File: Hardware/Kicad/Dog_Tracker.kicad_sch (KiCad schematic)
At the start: 20 parts, among them IC1 M4 Feather, U1 ADP160AUJZ-1.8-R7, U2 SX1280IMLTRT, U3 Origin_GPS1510, U4 NFA18SL407V1A45L, U5 SN74AUP1T97, U6 LSM6DSO32

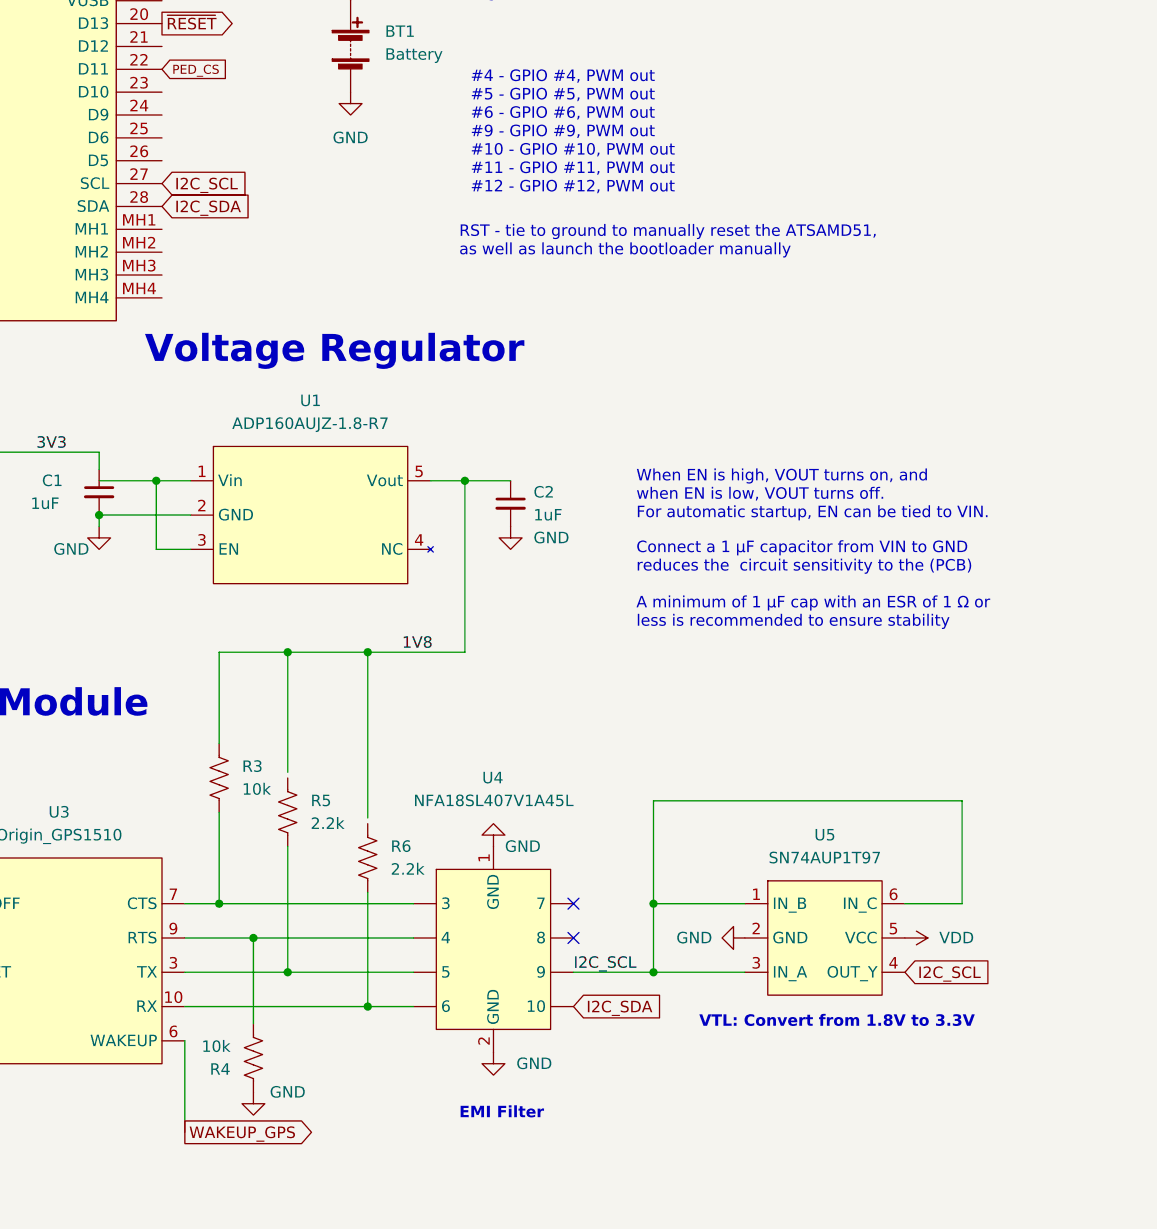
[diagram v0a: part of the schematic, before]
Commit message: 'wire i2c'
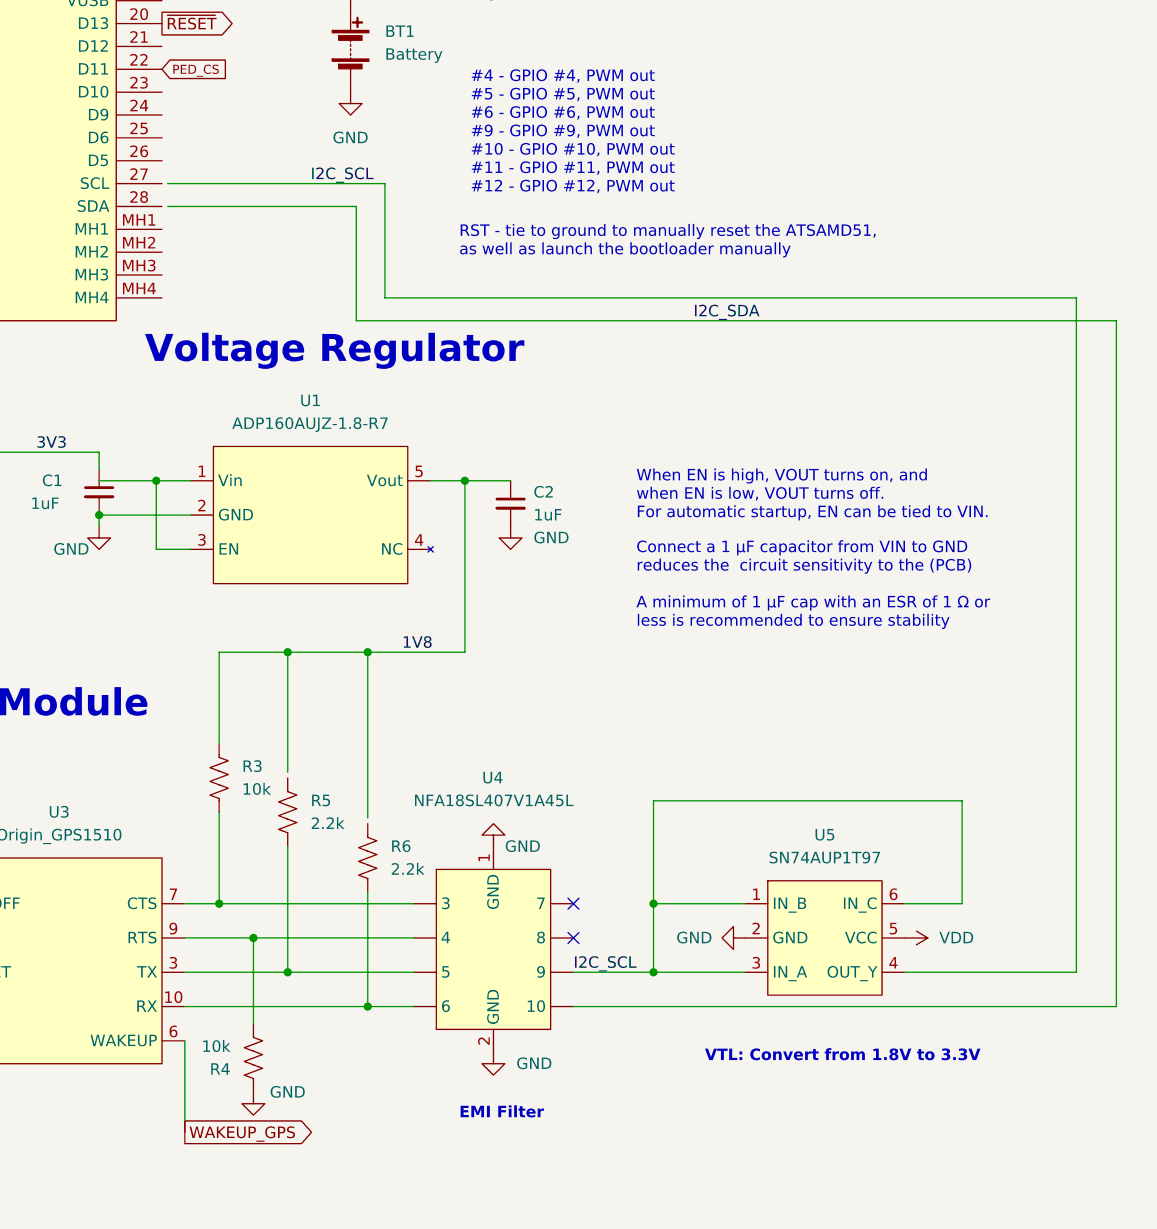
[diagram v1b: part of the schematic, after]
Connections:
- net I2C_SCL: no longer IC1.27 (SCL)
- net I2C_SDA: no longer IC1.28 (SDA)
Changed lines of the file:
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@@
+    (stroke (width 0) (type default) (color 0 0 0 0))
+  )
+  (wire (pts (xy 171.45 60.325) (xy 192.405 60.325))
     (stroke (width 0) (type default) (color 0 0 0 0))
   )
@@
     (stroke (width 0) (type default) (color 0 0 0 0))
   )
+  (wire (pts (xy 276.86 73.025) (xy 276.86 149.225))
+    (stroke (width 0) (type default) (color 0 0 0 0))
+  )
   (wire (pts (xy 121.285 47.625) (xy 121.285 75.565))
     (stroke (width 0) (type default) (color 0 0 0 0))
@@
     (stroke (width 0) (type default) (color 0 0 0 0))
   )
+  (wire (pts (xy 195.58 57.785) (xy 195.58 70.485))
+    (stroke (width 0) (type default) (color 0 0 0 0))
+  )
   (wire (pts (xy 184.785 123.19) (xy 184.785 109.855))
     (stroke (width 0) (type default) (color 0 0 0 0))
@@
     (stroke (width 0) (type default) (color 0 0 0 0))
   )
+  (wire (pts (xy 272.415 70.485) (xy 272.415 145.415))
+    (stroke (width 0) (type default) (color 0 0 0 0))
+  )
   (wire (pts (xy 259.715 137.795) (xy 253.365 137.795))
     (stroke (width 0) (type default) (color 0 0 0 0))
@@
     (stroke (width 0) (type default) (color 0 0 0 0))
   )
+  (wire (pts (xy 192.405 60.325) (xy 192.405 73.025))
+    (stroke (width 0) (type default) (color 0 0 0 0))
+  )
   (wire (pts (xy 95.25 80.645) (xy 118.11 80.645))
     (stroke (width 0) (type default) (color 0 0 0 0))
@@
     (stroke (width 0) (type default) (color 0 0 0 0))
   )
+  (wire (pts (xy 171.45 57.785) (xy 195.58 57.785))
+    (stroke (width 0) (type default) (color 0 0 0 0))
+  )
   (wire (pts (xy 130.175 87.63) (xy 163.83 87.63))
     (stroke (width 0) (type default) (color 0 0 0 0))
@@
     (stroke (width 0) (type default) (color 0 0 0 0))
   )
+  (wire (pts (xy 195.58 70.485) (xy 272.415 70.485))
+    (stroke (width 0) (type default) (color 0 0 0 0))
+  )
+  (wire (pts (xy 276.86 149.225) (xy 216.535 149.225))
+    (stroke (width 0) (type default) (color 0 0 0 0))
+  )
   (wire (pts (xy 128.905 34.925) (xy 128.905 47.625))
     (stroke (width 0) (type default) (color 0 0 0 0))
@@
     (stroke (width 0) (type default) (color 0 0 0 0))
   )
+  (wire (pts (xy 192.405 73.025) (xy 276.86 73.025))
+    (stroke (width 0) (type default) (color 0 0 0 0))
+  )
   (wire (pts (xy 81.915 40.005) (xy 114.935 40.005))
     (stroke (width 0) (type default) (color 0 0 0 0))
@@
   )
   (wire (pts (xy 102.235 63.5) (xy 102.235 70.485))
+    (stroke (width 0) (type default) (color 0 0 0 0))
+  )
+  (wire (pts (xy 272.415 145.415) (xy 253.365 145.415))
     (stroke (width 0) (type default) (color 0 0 0 0))
   )
@@
     (effects (font (size 1.27 1.27)) (justify left bottom))
   )
-  (text "VTL: Convert from 1.8V to 3.3V" (at 230.505 151.765 0)
+  (text "VTL: Convert from 1.8V to 3.3V" (at 231.14 155.575 0)
     (effects (font (size 1.27 1.27) (thickness 0.254) bold) (justify left bottom))
   )
@@
     (effects (font (size 1.27 1.27)) (justify left bottom))
   )
-  (global_label "I2C_SDA" (shape input) (at 216.535 149.225 0) (fields_autoplaced)
-    (effects (font (size 1.27 1.27)) (justify left))
-    (property "Intersheet References" "${INTERSHEET_REFS}" (id 0) (at 226.5681 149.1456 0)
-      (effects (font (size 1.27 1.27)) (justify left) hide)
-    )
+  (label "I2C_SCL" (at 187.325 57.785 0)
+    (effects (font (size 1.27 1.27)) (justify left bottom))
+  )
+  (label "I2C_SDA" (at 229.87 73.025 0)
+    (effects (font (size 1.27 1.27)) (justify left bottom))
   )
   (global_label "WAKEUP_GPS" (shape input) (at 140.335 52.705 180) (fields_autoplaced)
@@
     )
   )
-  (global_label "I2C_SCL" (shape input) (at 253.365 145.415 0) (fields_autoplaced)
-    (effects (font (size 1.27 1.27)) (justify left))
-    (property "Intersheet References" "${INTERSHEET_REFS}" (id 0) (at 263.3376 145.3356 0)
-      (effects (font (size 1.27 1.27)) (justify left) hide)
-    )
-  )
   (global_label "PED_CS" (shape input) (at 170.815 45.085 0) (fields_autoplaced)
     (effects (font (size 1 1)) (justify left))
@@
     )
   )
-  (global_label "I2C_SCL" (shape input) (at 170.815 57.785 0) (fields_autoplaced)
-    (effects (font (size 1.27 1.27)) (justify left))
-    (property "Intersheet References" "${INTERSHEET_REFS}" (id 0) (at 180.7876 57.7056 0)
-      (effects (font (size 1.27 1.27)) (justify left) hide)
-    )
-  )
   (global_label "~{RESET}" (shape output) (at 170.815 40.005 0) (fields_autoplaced)
     (effects (font (size 1.27 1.27)) (justify left))
@@
     )
   )
-  (global_label "I2C_SDA" (shape input) (at 170.815 60.325 0) (fields_autoplaced)
-    (effects (font (size 1.27 1.27)) (justify left))
-    (property "Intersheet References" "${INTERSHEET_REFS}" (id 0) (at 180.8481 60.2456 0)
-      (effects (font (size 1.27 1.27)) (justify left) hide)
-    )
-  )
